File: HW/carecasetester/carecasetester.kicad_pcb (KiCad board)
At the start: 2 copper layers, 158.3 x 160.4 mm, 72 parts, among them J1 Conn_01x16_Female, J10-TP22 Conn_01x01_Male, J11-TP7 Conn_01x01_Male, J12-TP14 Conn_01x01_Male, J13-TP23 Conn_01x01_Male, J14-TP17 Conn_01x01_Male, J15 Conn_01x16_Male, J15-TP1 Conn_01x01_Male, J15-TP20 Conn_01x01_Male, J16-TP2 Conn_01x01_Male, J16-TP24 Conn_01x01_Male, J17-TP3 Conn_01x01_Male, J18-TP4 Conn_01x01_Male, J19-TP6 Conn_01x01_Male, J2 Conn_01x16_Female, J20-TP9 Conn_01x01_Male, J21-TP10 Conn_01x01_Male, J22-TP11 Conn_01x01_Male, J23-TP12 Conn_01x01_Male, J24-TP15 Conn_01x01_Male, J25-TP18 Conn_01x01_Male, J26-TP5 Conn_01x01_Male, J27-TP26 Conn_01x01_Male, J3 Conn_01x04_Female, J4 Conn_01x06_Male, J4-TP16 Conn_01x01_Male, J5 12V_Psu, J5-TP8 Conn_01x01_Male, J5-~E1 Conn_01x02_Male, J6-TP21 Conn_01x01_Male, J7-TP27 Conn_01x01_Male, J8-TP13 Conn_01x01_Male, J9-TP19 Conn_01x01_Male, K1 AZ952, Q1 BC847, SW1 SW_DIP_x02, U1 CD74HC4067M, U2 L7805

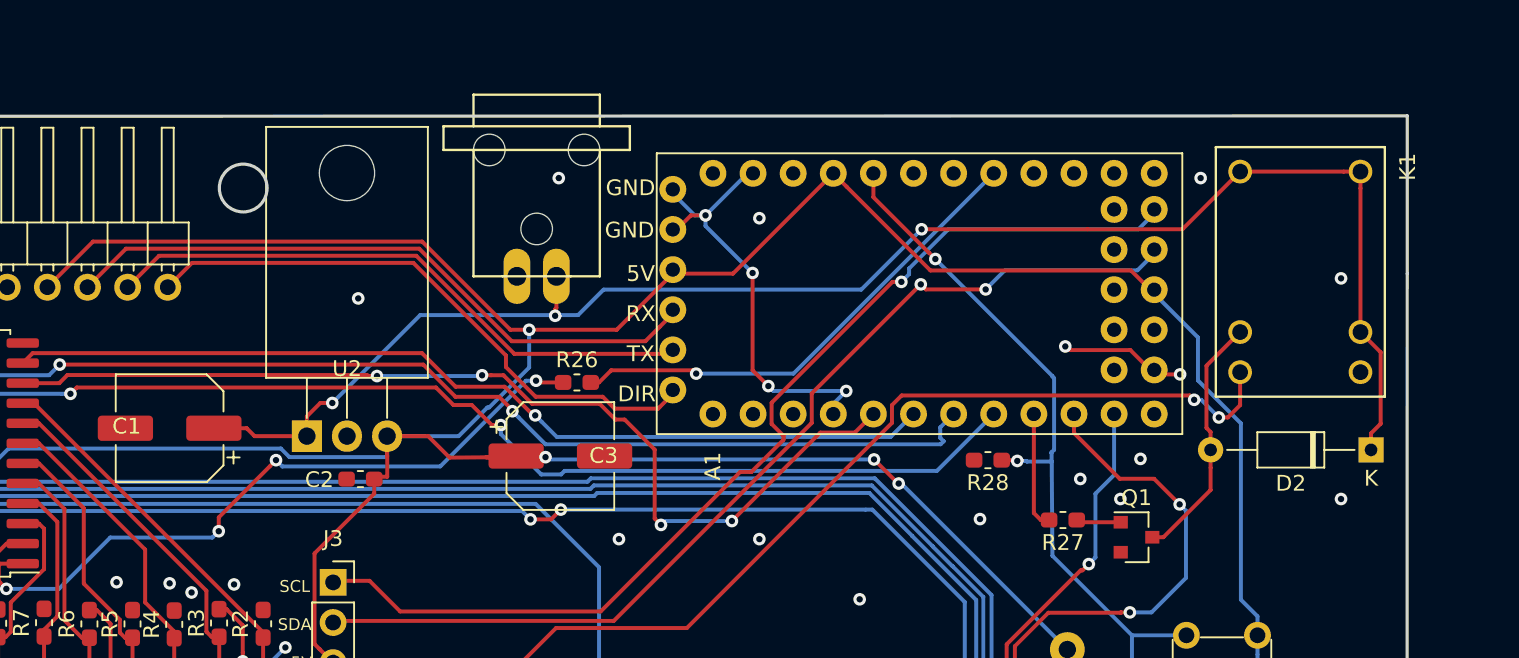
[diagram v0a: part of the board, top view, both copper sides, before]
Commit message: PCB and Schematic are synced and gerbers can be made
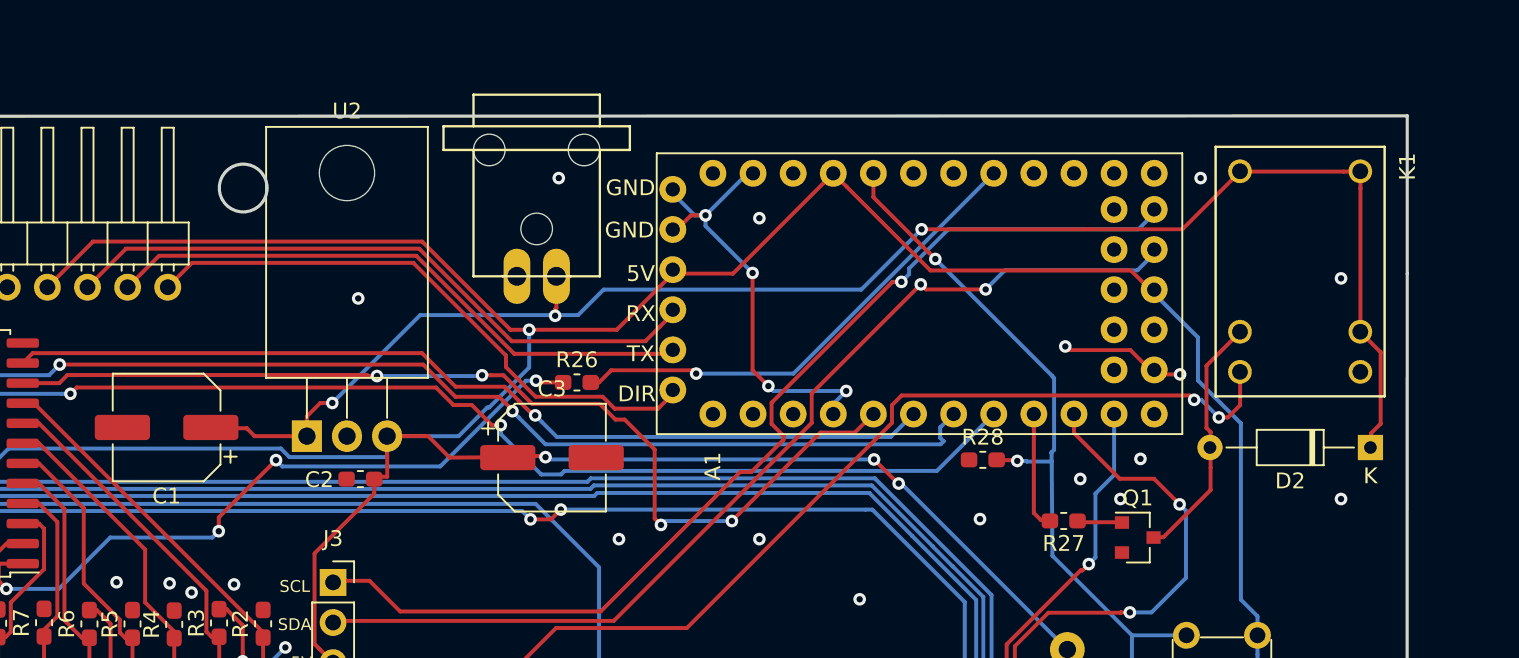
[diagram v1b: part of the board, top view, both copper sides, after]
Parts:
- Q1: value BC847 -> BC847W
- R28: value 4k7 -> 47k
- moved C3 0.54 mm to (181.2, 31.7)
- moved R28 0.32 mm to (208.5, 31.8), turned to 0 degrees
- moved C1 0.20 mm to (156.8, 29.8)
- moved D2 0.16 mm to (233.0, 31.0)
- moved Q1 0.08 mm to (218.3, 36.7)
- moved R27 0.08 mm to (213.6, 35.7)
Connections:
- net /RELAY/Relay_Driver renamed /RELAY/Relay_driver
- J5 pad 1: +12V -> GND
- J5 pad 2: GND -> +12V
- R28 pad 1: Net-(A1-Pad36) -> GND
- R28 pad 2: GND -> Net-(A1-Pad36)
